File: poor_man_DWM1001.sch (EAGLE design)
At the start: 18 parts, among them CN1 B2B-PH-K-S, IC1 E73_2G4M04S, Q3 MOSFET-NCHANNELSMD, U1 DWM1000_BREAKOUT, U3 MIC5205-3.3YM5-TR

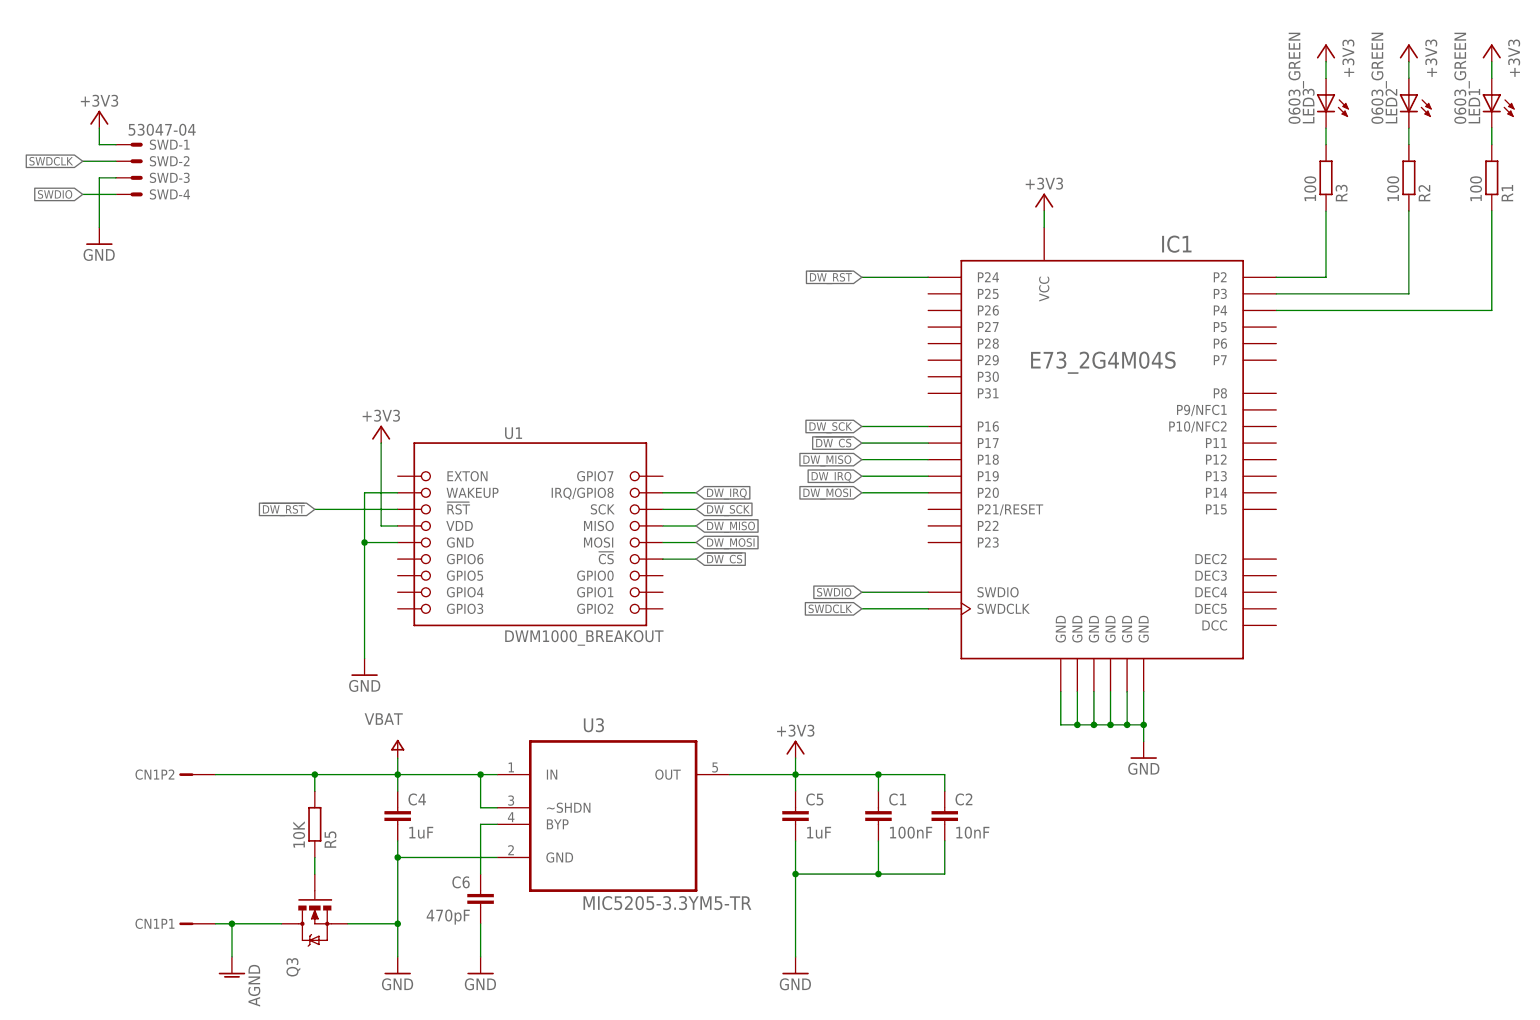
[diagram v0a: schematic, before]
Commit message: Daily save
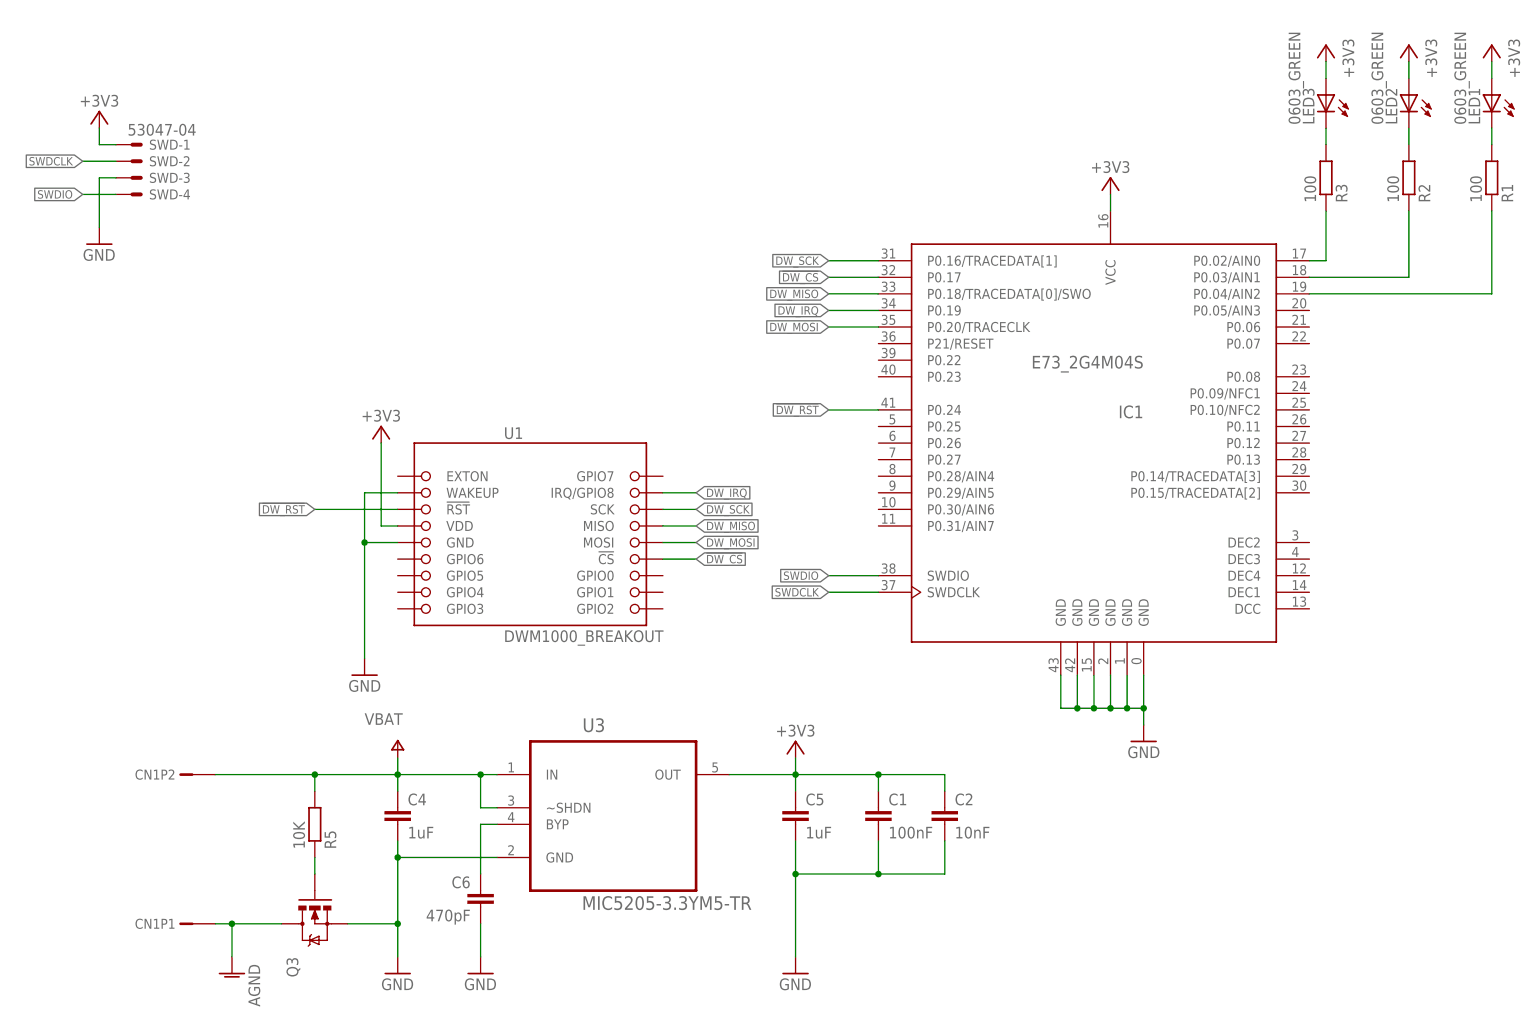
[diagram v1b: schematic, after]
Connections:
- net !DW_CS: now also IC1.P0.17; no longer IC1.P17
- net !DW_RST: now also IC1.P0.24; no longer IC1.P24
- net DW_IRQ: now also IC1.P0.19; no longer IC1.P19
- net DW_MISO: now also IC1.P0.18/TRACEDATA[0]/SWO; no longer IC1.P18
- net DW_MOSI: now also IC1.P0.20/TRACECLK; no longer IC1.P20
- net DW_SCK: now also IC1.P0.16/TRACEDATA[1]; no longer IC1.P16
- net N$4: now also IC1.P0.03/AIN1; no longer IC1.P3
- net N$5: now also IC1.P0.04/AIN2; no longer IC1.P4
- net N$6: now also IC1.P0.02/AIN0; no longer IC1.P2
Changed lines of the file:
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@@
 <parts>
 <part name="U1" library="martonmiklos" deviceset="DWM1000_BREAKOUT" device=""/>
-<part name="IC1" library="E73-2G4M04S" deviceset="E73_2G4M04S" device=""/>
 <part name="GND1" library="supply1" deviceset="GND" device=""/>
 <part name="+3V1" library="supply1" deviceset="+3V3" device=""/>
@@
 <part name="C1" library="rcl" deviceset="C-EU" device="C0603" value="100nF"/>
 <part name="C2" library="rcl" deviceset="C-EU" device="C0603" value="10nF"/>
+<part name="IC1" library="E73-2G4M04S" deviceset="E73_2G4M04S" device=""/>
 </parts>
 <sheets>
@@
 <instances>
 <instance part="U1" gate="G$1" x="86.36" y="91.44" rot="MR0"/>
-<instance part="IC1" gate="G$1" x="175.26" y="106.68" smashed="yes" rot="MR0">
-<attribute name="NAME" x="187.96" y="133.35" size="2.54" layer="95" rot="MR0"/>
-<attribute name="VALUE" x="185.42" y="115.57" size="2.54" layer="96" rot="MR0"/>
-</instance>
-<instance part="GND1" gate="1" x="180.34" y="55.88" rot="MR0"/>
-<instance part="+3V1" gate="G$1" x="165.1" y="142.24" rot="MR0"/>
+<instance part="GND1" gate="1" x="180.34" y="58.42" rot="MR0"/>
+<instance part="+3V1" gate="G$1" x="175.26" y="144.78" rot="MR0"/>
 <instance part="+3V2" gate="G$1" x="63.5" y="106.68" rot="MR0"/>
 <instance part="GND2" gate="1" x="60.96" y="68.58" rot="MR0"/>
@@
 <instance part="C1" gate="G$1" x="139.7" y="48.26"/>
 <instance part="C2" gate="G$1" x="149.86" y="48.26"/>
+<instance part="IC1" gate="G$1" x="175.26" y="109.22" rot="MR0"/>
 </instances>
 <busses>
@@
 <segment>
 <pinref part="GND1" gate="1" pin="GND"/>
+<wire x1="180.34" y1="60.96" x2="180.34" y2="63.5" width="0.1524" layer="91"/>
+<wire x1="180.34" y1="63.5" x2="180.34" y2="68.58" width="0.1524" layer="91"/>
+<wire x1="180.34" y1="63.5" x2="177.8" y2="63.5" width="0.1524" layer="91"/>
+<wire x1="177.8" y1="63.5" x2="177.8" y2="68.58" width="0.1524" layer="91"/>
+<junction x="180.34" y="63.5"/>
+<wire x1="177.8" y1="63.5" x2="175.26" y2="63.5" width="0.1524" layer="91"/>
+<wire x1="175.26" y1="63.5" x2="175.26" y2="68.58" width="0.1524" layer="91"/>
+<junction x="177.8" y="63.5"/>
+<wire x1="175.26" y1="63.5" x2="172.72" y2="63.5" width="0.1524" layer="91"/>
+<wire x1="172.72" y1="63.5" x2="172.72" y2="68.58" width="0.1524" layer="91"/>
+<junction x="175.26" y="63.5"/>
+<wire x1="172.72" y1="63.5" x2="170.18" y2="63.5" width="0.1524" layer="91"/>
+<wire x1="170.18" y1="63.5" x2="170.18" y2="68.58" width="0.1524" layer="91"/>
+<junction x="172.72" y="63.5"/>
+<wire x1="170.18" y1="63.5" x2="167.64" y2="63.5" width="0.1524" layer="91"/>
+<wire x1="167.64" y1="63.5" x2="167.64" y2="68.58" width="0.1524" layer="91"/>
+<junction x="170.18" y="63.5"/>
+<pinref part="IC1" gate="G$1" pin="GND@2"/>
 <pinref part="IC1" gate="G$1" pin="GND@1"/>
-<wire x1="180.34" y1="58.42" x2="180.34" y2="60.96" width="0.1524" layer="91"/>
-<pinref part="IC1" gate="G$1" pin="GND@2"/>
-<wire x1="180.34" y1="60.96" x2="180.34" y2="66.04" width="0.1524" layer="91"/>
-<wire x1="180.34" y1="60.96" x2="177.8" y2="60.96" width="0.1524" layer="91"/>
-<wire x1="177.8" y1="60.96" x2="177.8" y2="66.04" width="0.1524" layer="91"/>
-<junction x="180.34" y="60.96"/>
 <pinref part="IC1" gate="G$1" pin="GND@3"/>
-<wire x1="177.8" y1="60.96" x2="175.26" y2="60.96" width="0.1524" layer="91"/>
-<wire x1="175.26" y1="60.96" x2="175.26" y2="66.04" width="0.1524" layer="91"/>
-<junction x="177.8" y="60.96"/>
 <pinref part="IC1" gate="G$1" pin="GND@4"/>
-<wire x1="175.26" y1="60.96" x2="172.72" y2="60.96" width="0.1524" layer="91"/>
-<wire x1="172.72" y1="60.96" x2="172.72" y2="66.04" width="0.1524" layer="91"/>
-<junction x="175.26" y="60.96"/>
 <pinref part="IC1" gate="G$1" pin="GND@5"/>
-<wire x1="172.72" y1="60.96" x2="170.18" y2="60.96" width="0.1524" layer="91"/>
-<wire x1="170.18" y1="60.96" x2="170.18" y2="66.04" width="0.1524" layer="91"/>
-<junction x="172.72" y="60.96"/>
 <pinref part="IC1" gate="G$1" pin="GND@6"/>
-<wire x1="170.18" y1="60.96" x2="167.64" y2="60.96" width="0.1524" layer="91"/>
-<wire x1="167.64" y1="60.96" x2="167.64" y2="66.04" width="0.1524" layer="91"/>
-<junction x="170.18" y="60.96"/>
 </segment>
 <segment>
@@
 </net>
 <net name="+3V3" class="0">
-<segment>
-<pinref part="IC1" gate="G$1" pin="VCC@1"/>
-<pinref part="+3V1" gate="G$1" pin="+3V3"/>
-<wire x1="165.1" y1="139.7" x2="165.1" y2="137.16" width="0.1524" layer="91"/>
-</segment>
 <segment>
 <pinref part="U1" gate="G$1" pin="VDD"/>
@@
 <wire x1="149.86" y1="53.34" x2="149.86" y2="50.8" width="0.1524" layer="91"/>
 </segment>
+<segment>
+<pinref part="+3V1" gate="G$1" pin="+3V3"/>
+<pinref part="IC1" gate="G$1" pin="VCC@1"/>
+<wire x1="175.26" y1="142.24" x2="175.26" y2="139.7" width="0.1524" layer="91"/>
+</segment>
 </net>
 <net name="!DW_CS" class="0">
@@
 </segment>
 <segment>
-<pinref part="IC1" gate="G$1" pin="P17"/>
-<wire x1="147.32" y1="104.14" x2="137.16" y2="104.14" width="0.1524" layer="91"/>
-<label x="137.16" y="104.14" size="1.27" layer="95" font="vector" rot="MR0" xref="yes"/>
+<wire x1="139.7" y1="129.54" x2="132.08" y2="129.54" width="0.1524" layer="91"/>
+<label x="132.08" y="129.54" size="1.27" layer="95" font="vector" rot="MR0" xref="yes"/>
+<pinref part="IC1" gate="G$1" pin="P0.17"/>
 </segment>
 </net>
@@
 </segment>
 <segment>
-<pinref part="IC1" gate="G$1" pin="P24"/>
-<wire x1="147.32" y1="129.54" x2="137.16" y2="129.54" width="0.1524" layer="91"/>
-<label x="137.16" y="129.54" size="1.27" layer="95" font="vector" rot="R180" xref="yes"/>
+<wire x1="139.7" y1="109.22" x2="132.08" y2="109.22" width="0.1524" layer="91"/>
+<label x="132.08" y="109.22" size="1.27" layer="95" font="vector" rot="R180" xref="yes"/>
+<pinref part="IC1" gate="G$1" pin="P0.24"/>
 </segment>
 </net>
@@
 </segment>
 <segment>
-<pinref part="IC1" gate="G$1" pin="P16"/>
-<wire x1="147.32" y1="106.68" x2="137.16" y2="106.68" width="0.1524" layer="91"/>
-<label x="137.16" y="106.68" size="1.27" layer="95" font="vector" rot="MR0" xref="yes"/>
+<wire x1="139.7" y1="132.08" x2="132.08" y2="132.08" width="0.1524" layer="91"/>
+<label x="132.08" y="132.08" size="1.27" layer="95" font="vector" rot="MR0" xref="yes"/>
+<pinref part="IC1" gate="G$1" pin="P0.16/TRACEDATA[1]"/>
 </segment>
 </net>
@@
 </segment>
 <segment>
-<pinref part="IC1" gate="G$1" pin="P18"/>
-<wire x1="147.32" y1="101.6" x2="137.16" y2="101.6" width="0.1524" layer="91"/>
-<label x="137.16" y="101.6" size="1.27" layer="95" font="vector" rot="MR0" xref="yes"/>
+<wire x1="139.7" y1="127" x2="132.08" y2="127" width="0.1524" layer="91"/>
+<label x="132.08" y="127" size="1.27" layer="95" font="vector" rot="MR0" xref="yes"/>
+<pinref part="IC1" gate="G$1" pin="P0.18/TRACEDATA[0]/SWO"/>
 </segment>
 </net>
@@
 </segment>
 <segment>
-<pinref part="IC1" gate="G$1" pin="P20"/>
-<wire x1="147.32" y1="96.52" x2="137.16" y2="96.52" width="0.1524" layer="91"/>
-<label x="137.16" y="96.52" size="1.27" layer="95" font="vector" rot="MR0" xref="yes"/>
+<wire x1="139.7" y1="121.92" x2="132.08" y2="121.92" width="0.1524" layer="91"/>
+<label x="132.08" y="121.92" size="1.27" layer="95" font="vector" rot="MR0" xref="yes"/>
+<pinref part="IC1" gate="G$1" pin="P0.20/TRACECLK"/>
 </segment>
 </net>
@@
 </segment>
 <segment>
-<pinref part="IC1" gate="G$1" pin="P19"/>
-<wire x1="147.32" y1="99.06" x2="137.16" y2="99.06" width="0.1524" layer="91"/>
-<label x="137.16" y="99.06" size="1.27" layer="95" font="vector" rot="MR0" xref="yes"/>
+<wire x1="139.7" y1="124.46" x2="132.08" y2="124.46" width="0.1524" layer="91"/>
+<label x="132.08" y="124.46" size="1.27" layer="95" font="vector" rot="MR0" xref="yes"/>
+<pinref part="IC1" gate="G$1" pin="P0.19"/>
 </segment>
 </net>
@@
 </segment>
 <segment>
+<wire x1="139.7" y1="81.28" x2="132.08" y2="81.28" width="0.1524" layer="91"/>
+<label x="132.08" y="81.28" size="1.27" layer="95" font="vector" rot="MR0" xref="yes"/>
 <pinref part="IC1" gate="G$1" pin="SWDCLK"/>
-<wire x1="147.32" y1="78.74" x2="137.16" y2="78.74" width="0.1524" layer="91"/>
-<label x="137.16" y="78.74" size="1.27" layer="95" font="vector" rot="MR0" xref="yes"/>
 </segment>
 </net>
@@
 </segment>
 <segment>
+<wire x1="139.7" y1="83.82" x2="132.08" y2="83.82" width="0.1524" layer="91"/>
+<label x="132.08" y="83.82" size="1.27" layer="95" font="vector" rot="MR0" xref="yes"/>
 <pinref part="IC1" gate="G$1" pin="SWDIO"/>
-<wire x1="147.32" y1="81.28" x2="137.16" y2="81.28" width="0.1524" layer="91"/>
-<label x="137.16" y="81.28" size="1.27" layer="95" font="vector" rot="MR0" xref="yes"/>
 </segment>
 </net>
@@
 <segment>
 <pinref part="R2" gate="G$1" pin="1"/>
-<pinref part="IC1" gate="G$1" pin="P3"/>
-<wire x1="200.66" y1="127" x2="220.98" y2="127" width="0.1524" layer="91"/>
-<wire x1="220.98" y1="127" x2="220.98" y2="139.7" width="0.1524" layer="91"/>
+<wire x1="205.74" y1="129.54" x2="220.98" y2="129.54" width="0.1524" layer="91"/>
+<wire x1="220.98" y1="129.54" x2="220.98" y2="139.7" width="0.1524" layer="91"/>
+<pinref part="IC1" gate="G$1" pin="P0.03/AIN1"/>
 </segment>
 </net>
@@
 <segment>
 <pinref part="R1" gate="G$1" pin="1"/>
-<pinref part="IC1" gate="G$1" pin="P4"/>
-<wire x1="200.66" y1="124.46" x2="233.68" y2="124.46" width="0.1524" layer="91"/>
-<wire x1="233.68" y1="124.46" x2="233.68" y2="139.7" width="0.1524" layer="91"/>
+<wire x1="205.74" y1="127" x2="233.68" y2="127" width="0.1524" layer="91"/>
+<wire x1="233.68" y1="127" x2="233.68" y2="139.7" width="0.1524" layer="91"/>
+<pinref part="IC1" gate="G$1" pin="P0.04/AIN2"/>
 </segment>
 </net>
@@
 <segment>
 <pinref part="R3" gate="G$1" pin="1"/>
-<pinref part="IC1" gate="G$1" pin="P2"/>
-<wire x1="200.66" y1="129.54" x2="208.28" y2="129.54" width="0.1524" layer="91"/>
-<wire x1="208.28" y1="129.54" x2="208.28" y2="139.7" width="0.1524" layer="91"/>
-</segment>
-</net>
+<wire x1="205.74" y1="132.08" x2="208.28" y2="132.08" width="0.1524" layer="91"/>
+<wire x1="208.28" y1="132.08" x2="208.28" y2="139.7" width="0.1524" layer="91"/>
+<pinref part="IC1" gate="G$1" pin="P0.02/AIN0"/>
+</segment>
+</net>

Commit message: - Updated net names
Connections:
- net N$1 renamed GPIO_LED1_R
- net N$2 renamed GPIO_LED2_R
- net N$3 renamed GPIO_LED3_R
- net N$4 renamed GPIO_LED2
- net N$5 renamed GPIO_LED1
- net N$6 renamed GPIO_LED3
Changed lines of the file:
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@@
 <?xml version="1.0" encoding="utf-8"?>
 <!DOCTYPE eagle SYSTEM "eagle.dtd">
-<eagle version="8.7.0">
+<eagle version="9.0.0">
 <drawing>
 <settings>
@@
 </segment>
 </net>
-<net name="N$1" class="0">
+<net name="GPIO_LED1_R" class="0">
 <segment>
 <pinref part="R1" gate="G$1" pin="2"/>
@@
 </segment>
 </net>
-<net name="N$2" class="0">
+<net name="GPIO_LED2_R" class="0">
 <segment>
 <pinref part="R2" gate="G$1" pin="2"/>
@@
 </segment>
 </net>
-<net name="N$3" class="0">
+<net name="GPIO_LED3_R" class="0">
 <segment>
 <pinref part="R3" gate="G$1" pin="2"/>
@@
 </segment>
 </net>
-<net name="N$4" class="0">
+<net name="GPIO_LED2" class="0">
 <segment>
 <pinref part="R2" gate="G$1" pin="1"/>
@@
 </segment>
 </net>
-<net name="N$5" class="0">
+<net name="GPIO_LED1" class="0">
 <segment>
 <pinref part="R1" gate="G$1" pin="1"/>
@@
 </segment>
 </net>
-<net name="N$6" class="0">
+<net name="GPIO_LED3" class="0">
 <segment>
 <pinref part="R3" gate="G$1" pin="1"/>
